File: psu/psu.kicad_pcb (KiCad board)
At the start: 2 copper layers, 6 parts, among them J1 26-60-4023, J2 26-60-4023

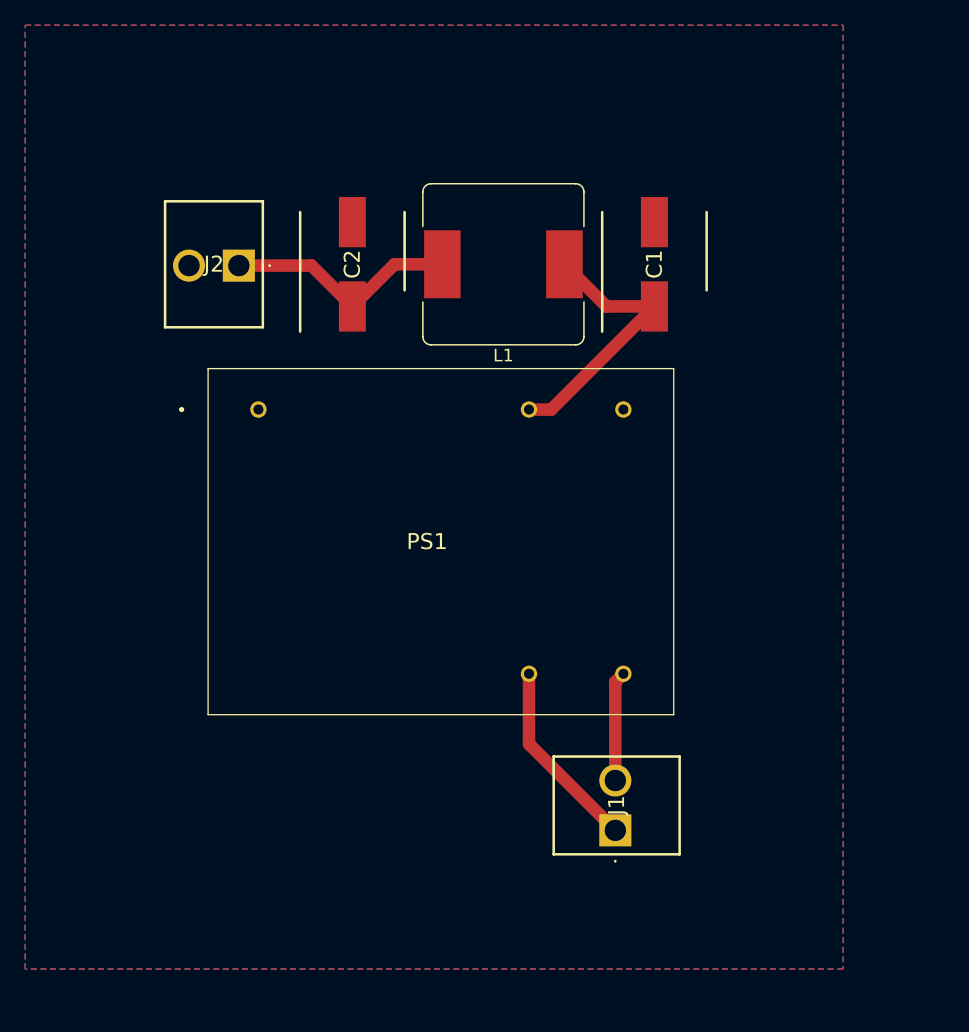
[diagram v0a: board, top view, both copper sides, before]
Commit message: likely all done with v1, mainboard obsolete
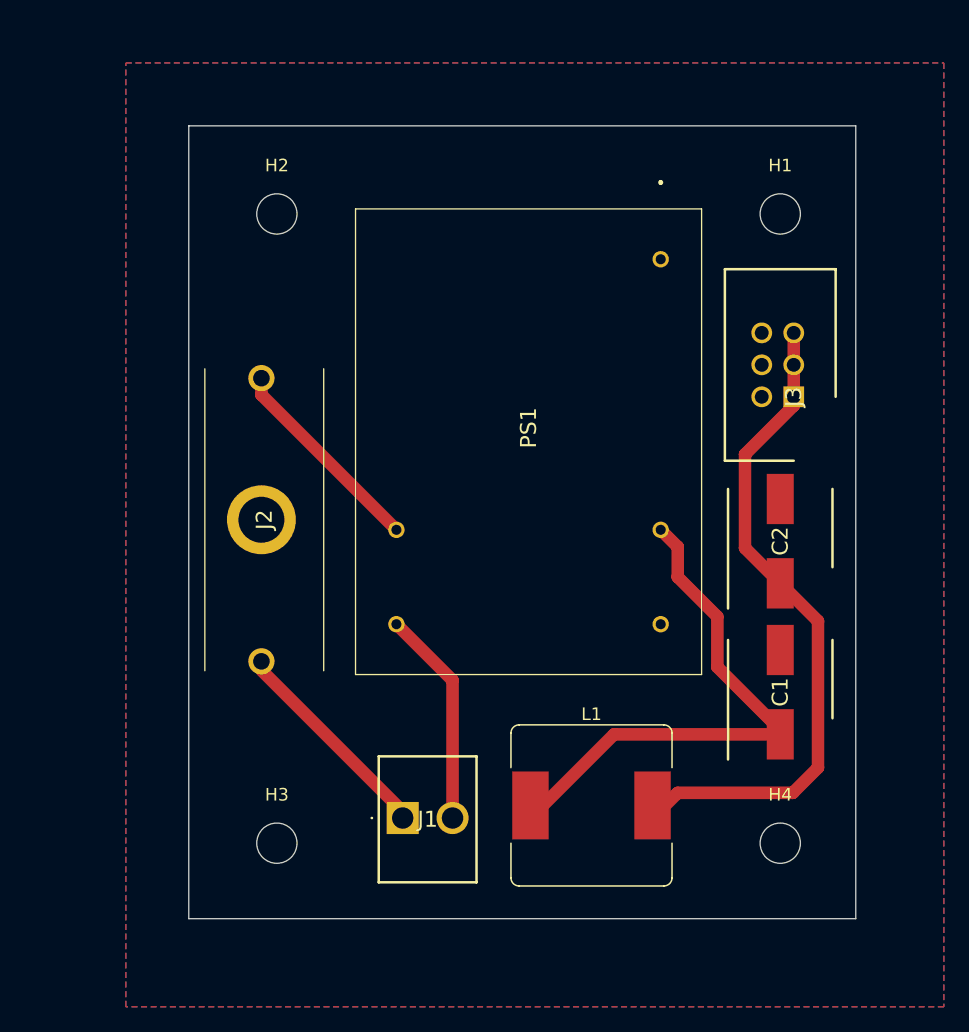
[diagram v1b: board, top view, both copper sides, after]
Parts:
- added H1: MountingHole, MountingHole:MountingHole_3.2mm_M3_ISO7380, F.Cu at (160.0, 45.0)
- added H2: MountingHole, MountingHole:MountingHole_3.2mm_M3_ISO7380, F.Cu at (120.0, 45.0)
- added H3: MountingHole, MountingHole:MountingHole_3.2mm_M3_ISO7380, F.Cu at (120.0, 95.0)
- added H4: MountingHole, MountingHole:MountingHole_3.2mm_M3_ISO7380, F.Cu at (160.0, 95.0)
- added J3: BHR-06-VUA, Samacsys:SHDR6W64P254_2X3_1522X880X920P, F.Cu at (161.1, 59.5)
- J2: value 26-60-4023 -> 4628; footprint Samacsys:26604023 -> Samacsys:4628
- moved L1 43.6 mm to (145.0, 92.0), turned to 0 degrees
- moved C2 40.5 mm to (160.0, 71.0)
- moved C1 35.4 mm to (160.0, 83.0)
- moved PS1 34.1 mm to (150.5, 48.6), turned to -90 degrees
- moved J2 31.5 mm to (118.8, 80.6), turned to 90 degrees
- moved J1 16.9 mm to (130.0, 93.0), turned to 180 degrees
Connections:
- J1 pad 1: Net-(PS1-AC_IN_(N)) -> Net-(J1-Pad1)
- J2 pad 1: +5V -> Net-(J1-Pad1)
- J2 pad 2: GNDD -> Net-(PS1-AC_IN_(N))
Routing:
- net +5V: track 18.9 -> 53.4 mm
- net Net-(C1-+): track 21.9 -> 42.8 mm
- net Net-(J1-Pad1): track 0.00 -> 16.4 mm
- net Net-(PS1-AC_IN_(L)): track 8.75 -> 17.2 mm
- net Net-(PS1-AC_IN_(N)): track 15.3 -> 15.8 mm
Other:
- board outline added: 53 x 63 mm
